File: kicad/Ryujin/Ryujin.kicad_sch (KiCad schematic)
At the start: 35 parts, among them J1 Conn_01x02_Socket, J10 Conn_01x04_Pin, J11 Conn_01x04_Pin, J12 Conn_01x04_Pin, J2 1822972, J3 Conn_01x14_Socket, J4 Conn_01x14_Socket, J5 1822972, J6 Conn_01x04_Pin, J7 Conn_01x04_Pin, J8 Conn_01x04_Pin, J9 Conn_01x04_Pin, Q1 IRLML5203, Q2 IRLML6244, U1 74LVC1G17, U2 74AHCT1G14, U3 TMUX1119DBVR, U4 SHTC3, U5 W25Q32JVSS, U7 R-78E5.0-1.0

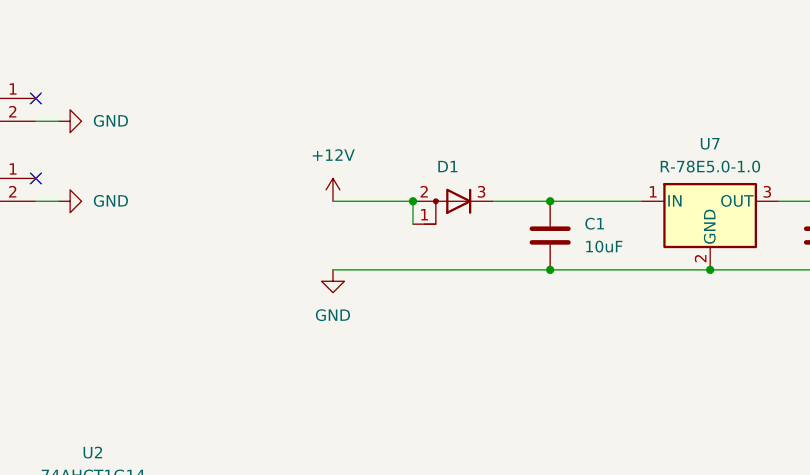
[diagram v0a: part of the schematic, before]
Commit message: A Tale of Two Muses
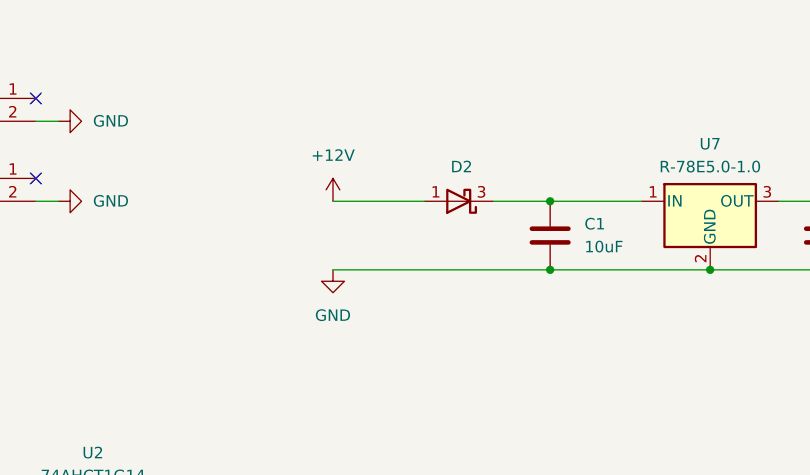
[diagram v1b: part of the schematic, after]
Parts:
- removed D8: D1, footprints:PDS104013, symbol Device:D_AAK
- added D8: D2, Package_TO_SOT_SMD:SOT-23, symbol Diode:BAT54W
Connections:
- net +12V: now also D8.1 (A)
- net at C1.1, U7.1 (IN): now also D8.3 (K)
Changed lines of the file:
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@@
 	)
 	(junction
-		(at 129.54 30.48)
-		(diameter 0)
-		(color 0 0 0 0)
-	)
-	(junction
 		(at 224.79 138.43)
 		(diameter 0)
@@
 	(wire
 		(pts
-			(xy 129.54 30.48) (xy 129.54 33.02)
-		)
-		(stroke
-			(width 0)
-			(type default)
-		)
-	)
-	(wire
-		(pts
 			(xy 50.8 29.21) (xy 50.8 26.67)
 		)
@@
 	(wire
 		(pts
-			(xy 120.65 30.48) (xy 129.54 30.48)
+			(xy 120.65 30.48) (xy 130.81 30.48)
 		)
 		(stroke
@@
 	)
 	(symbol
-		(lib_id "Device:D_AAK")
-		(at 134.62 30.48 180)
-		(unit 1)
-		(exclude_from_sim no)
-		(in_bom yes)
-		(on_board yes)
-		(dnp no)
-		(fields_autoplaced yes)
-		(property "Reference" "D8"
-			(at 133.4135 24.13 0)
-			(effects
-				(font
-					(size 1.27 1.27)
-				)
-				(hide yes)
-			)
-		)
-		(property "Value" "D1"
-			(at 133.4135 26.67 0)
-			(effects
-				(font
-					(size 1.27 1.27)
-				)
-			)
-		)
-		(property "Footprint" "footprints:PDS104013"
-			(at 134.62 30.48 0)
-			(effects
-				(font
-					(size 1.27 1.27)
-				)
-				(hide yes)
-			)
-		)
-		(property "Datasheet" "../../docs/PDS1040.pdf"
-			(at 134.62 30.48 0)
-			(effects
-				(font
-					(size 1.27 1.27)
-				)
-				(hide yes)
-			)
-		)
-		(property "Description" "Diode, anode on pins 1 and 2"
-			(at 134.62 30.48 0)
-			(effects
-				(font
-					(size 1.27 1.27)
-				)
-				(hide yes)
-			)
-		)
-		(property "MPN" "PDS1040-13"
-			(at 134.62 30.48 0)
-			(effects
-				(font
-					(size 1.27 1.27)
-				)
-				(hide yes)
-			)
-		)
-		(pin "3"
-		)
-		(pin "2"
-		)
-		(pin "1"
-		)
-		(instances
-			(project "Ryujin"
-				(path "/a03941d3-2006-4bae-a82d-663063c77238"
-					(reference "D8")
-					(unit 1)
-				)
-			)
-		)
-	)
-	(symbol
 		(lib_id "power:GND")
 		(at 177.8 92.71 0)
@@
 					(unit 1)
 				)
+			)
+		)
+	)
+	(symbol
+		(lib_id "Diode:BAT54W")
+		(at 134.62 30.48 180)
+		(unit 1)
+		(exclude_from_sim no)
+		(in_bom yes)
+		(on_board yes)
+		(dnp no)
+		(fields_autoplaced yes)
+		(property "Reference" "D8"
+			(at 136.2076 33.02 90)
+			(effects
+				(font
+					(size 1.27 1.27)
+				)
+				(justify left)
+				(hide yes)
+			)
+		)
+		(property "Value" "D2"
+			(at 134.9375 26.67 0)
+			(effects
+				(font
+					(size 1.27 1.27)
+				)
+			)
+		)
+		(property "Footprint" "Package_TO_SOT_SMD:SOT-23"
+			(at 134.62 26.035 0)
+			(effects
+				(font
+					(size 1.27 1.27)
+				)
+				(hide yes)
+			)
+		)
+		(property "Datasheet" "https://assets.nexperia.com/documents/data-sheet/BAT54W_SER.pdf"
+			(at 134.62 30.48 0)
+			(effects
+				(font
+					(size 1.27 1.27)
+				)
+				(hide yes)
+			)
+		)
+		(property "Description" "Schottky barrier diode"
+			(at 134.62 30.48 0)
+			(effects
+				(font
+					(size 1.27 1.27)
+				)
+				(hide yes)
+			)
+		)
+		(property "MPN" " BAT54"
+			(at 134.62 30.48 90)
+			(effects
+				(font
+					(size 1.27 1.27)
+				)
+				(hide yes)
+			)
+		)
+		(pin "1"
+		)
+		(pin "2"
+		)
+		(pin "3"
+		)
+		(instances
+			(project "Ryujin"
+				(path "/a03941d3-2006-4bae-a82d-663063c77238"
+					(reference "D8")
+					(unit 1)
+				)
